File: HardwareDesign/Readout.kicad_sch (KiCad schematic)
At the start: 4 parts, among them U2 74ACT163, U3 74ACT163, U4 74ACT163, U5 74ACT163

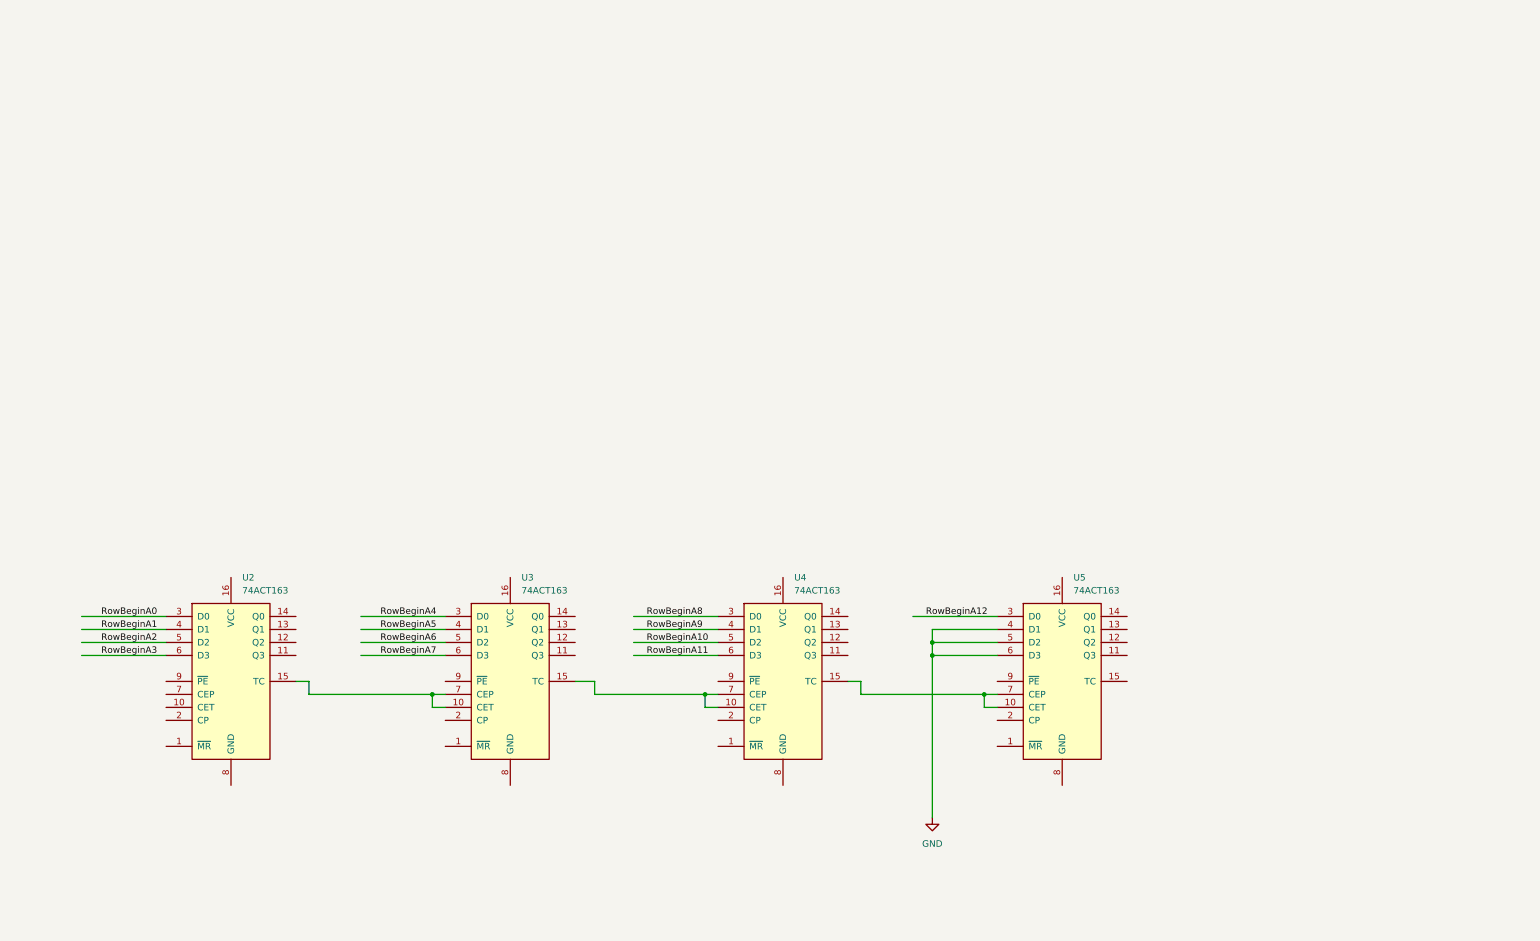
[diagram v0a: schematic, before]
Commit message: working on Readout module
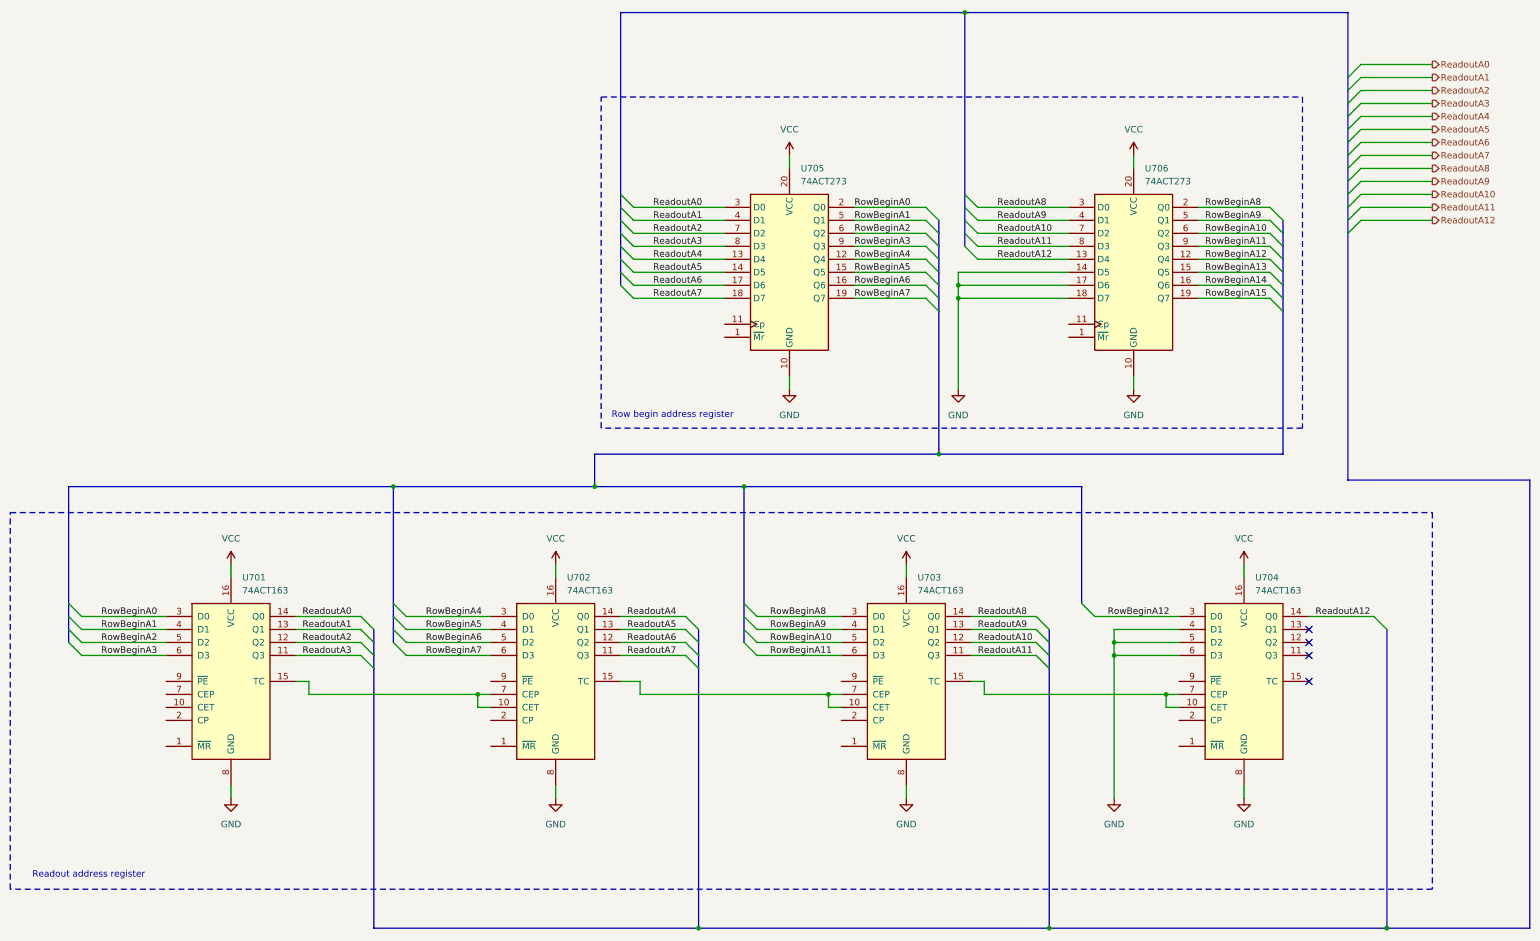
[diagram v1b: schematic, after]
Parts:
- added U705, U706: 74ACT273, symbol 74xx:74LS273
- renumbered U2 to U701, U3 to U702, U4 to U703, U5 to U704
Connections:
- net GND: now also U701.8 (GND), U702.8 (GND), U703.8 (GND), U704.8 (GND), U705.10 (GND), U706.10 (GND), U706.14 (D5), U706.17 (D6), U706.18 (D7)
- net RowBeginA0: now also U705.2 (Q0)
- net RowBeginA1: now also U705.5 (Q1)
- net RowBeginA10: now also U706.6 (Q2)
- net RowBeginA11: now also U706.9 (Q3)
- net RowBeginA12: now also U706.12 (Q4)
- net RowBeginA2: now also U705.6 (Q2)
- net RowBeginA3: now also U705.9 (Q3)
- net RowBeginA4: now also U705.12 (Q4)
- net RowBeginA5: now also U705.15 (Q5)
- net RowBeginA6: now also U705.16 (Q6)
- net RowBeginA7: now also U705.19 (Q7)
- net RowBeginA8: now also U706.2 (Q0)
- net RowBeginA9: now also U706.5 (Q1)
- net ReadoutA7: now reaches U702.11 (Q3)
- net ReadoutA7: now also U705.18 (D7)
- net ReadoutA6: now reaches U702.12 (Q2)
- net ReadoutA6: now also U705.17 (D6)
- net ReadoutA5: now reaches U702.13 (Q1)
- net ReadoutA5: now also U705.14 (D5)
- net ReadoutA4: now reaches U702.14 (Q0)
- net ReadoutA4: now also U705.13 (D4)
- net VCC: now reaches U702.16 (VCC)
- net VCC: now also U701.16 (VCC), U703.16 (VCC), U704.16 (VCC), U705.20 (VCC), U706.20 (VCC)
- net ReadoutA11: now reaches U703.11 (Q3)
- net ReadoutA11: now also U706.8 (D3)
- net ReadoutA10: now reaches U703.12 (Q2)
- net ReadoutA10: now also U706.7 (D2)
- net ReadoutA9: now reaches U703.13 (Q1)
- net ReadoutA9: now also U706.4 (D1)
- net ReadoutA8: now reaches U703.14 (Q0)
- net ReadoutA8: now also U706.3 (D0)
- net ReadoutA3: now reaches U701.11 (Q3)
- net ReadoutA3: now also U705.8 (D3)
- net ReadoutA2: now reaches U701.12 (Q2)
- net ReadoutA2: now also U705.7 (D2)
- net ReadoutA1: now reaches U701.13 (Q1)
- net ReadoutA1: now also U705.4 (D1)
- net ReadoutA0: now reaches U701.14 (Q0)
- net ReadoutA0: now also U705.3 (D0)
- net ReadoutA12: now reaches U704.14 (Q0)
- net ReadoutA12: now also U706.13 (D4)
- new net RowBeginA13: U706.15 (Q5)
- new net RowBeginA14: U706.16 (Q6)
- new net RowBeginA15: U706.19 (Q7)
- no-connect marks 0 -> 4
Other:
- note added: "Readout address register"
- note added: "Row begin address register"
- moved on the sheet: U702, U703, U704
